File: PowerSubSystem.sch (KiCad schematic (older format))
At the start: 14 parts, among them U401 LM3671

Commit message: lib update so it only includes user-made library
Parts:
- C401, C402, C404, C405, C406, C408, C409, C410: symbol BeagleBone-Black-Cape-rescue:C-Device -> UserMade-BB-Zigbee-Gateway-CAPE:C-Device
- C403, C407: symbol BeagleBone-Black-Cape-rescue:C_Small-Device -> UserMade-BB-Zigbee-Gateway-CAPE:C_Small-Device
- FB401: symbol BeagleBone-Black-Cape-rescue:Ferrite_Bead_Small-Device -> UserMade-BB-Zigbee-Gateway-CAPE:Ferrite_Bead_Small-Device
- L401: symbol BeagleBone-Black-Cape-rescue:L_Small-Device -> UserMade-BB-Zigbee-Gateway-CAPE:L_Small-Device
- L402: symbol BeagleBone-Black-Cape-rescue:INDUCTOR-pspice -> UserMade-BB-Zigbee-Gateway-CAPE:INDUCTOR-pspice
- U401: symbol pwr_BeagleBone:LM3671 -> UserMade-BB-Zigbee-Gateway-CAPE:LM3671
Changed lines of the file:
@@
 5Vin+ Comes from the 5V output \nof the beaglebone. The one \nthat is connected to the 12V \ninput.
 $Comp
-L pwr_BeagleBone:LM3671 U401
+L UserMade-BB-Zigbee-Gateway-CAPE:LM3671 U401
 U 1 1 613D6B2B
 P 3600 6150
@@
 $EndComp
 $Comp
-L BeagleBone-Black-Cape-rescue:C_Small-Device C403
+L UserMade-BB-Zigbee-Gateway-CAPE:C_Small-Device C403
 U 1 1 613D8B5E
 P 2950 6550
@@
 	3150 6500 3150 6800
 $Comp
-L BeagleBone-Black-Cape-rescue:L_Small-Device L401
+L UserMade-BB-Zigbee-Gateway-CAPE:L_Small-Device L401
 U 1 1 613E2221
 P 4150 6300
@@
 	4350 6500 4350 6300
 $Comp
-L BeagleBone-Black-Cape-rescue:GND-power #PWR0404
+L UserMade-BB-Zigbee-Gateway-CAPE:GND-power #PWR0404
 U 1 1 613E4C24
 P 2950 6900
@@
 	2950 6900 2950 6800
 $Comp
-L BeagleBone-Black-Cape-rescue:C_Small-Device C407
+L UserMade-BB-Zigbee-Gateway-CAPE:C_Small-Device C407
 U 1 1 613E66FD
 P 4600 6550
@@
 $EndComp
 $Comp
-L BeagleBone-Black-Cape-rescue:GND-power #PWR0408
+L UserMade-BB-Zigbee-Gateway-CAPE:GND-power #PWR0408
 U 1 1 613EB575
 P 4600 6900
@@
 Connection ~ 3150 6800
 $Comp
-L pwr_BeagleBone:SYS_5V #PWR0402
+L UserMade-BB-Zigbee-Gateway-CAPE:SYS_5V #PWR0402
 U 1 1 614A8F35
 P 2600 6300
@@
 VDDR
 $Comp
-L BeagleBone-Black-Cape-rescue:C-Device C402
+L UserMade-BB-Zigbee-Gateway-CAPE:C-Device C402
 U 1 1 614ACFF1
 P 2800 2950
@@
 $EndComp
 $Comp
-L BeagleBone-Black-Cape-rescue:C-Device C401
+L UserMade-BB-Zigbee-Gateway-CAPE:C-Device C401
 U 1 1 614AD67F
 P 2300 2950
@@
 $EndComp
 $Comp
-L BeagleBone-Black-Cape-rescue:C-Device C409
+L UserMade-BB-Zigbee-Gateway-CAPE:C-Device C409
 U 1 1 614ADB54
 P 8450 2950
@@
 $EndComp
 $Comp
-L BeagleBone-Black-Cape-rescue:C-Device C406
+L UserMade-BB-Zigbee-Gateway-CAPE:C-Device C406
 U 1 1 614ADE06
 P 4350 2950
@@
 $EndComp
 $Comp
-L BeagleBone-Black-Cape-rescue:C-Device C404
+L UserMade-BB-Zigbee-Gateway-CAPE:C-Device C404
 U 1 1 614ADFDD
 P 3300 2950
@@
 $EndComp
 $Comp
-L BeagleBone-Black-Cape-rescue:C-Device C410
+L UserMade-BB-Zigbee-Gateway-CAPE:C-Device C410
 U 1 1 614AE392
 P 8950 2950
@@
 $EndComp
 $Comp
-L BeagleBone-Black-Cape-rescue:C-Device C405
+L UserMade-BB-Zigbee-Gateway-CAPE:C-Device C405
 U 1 1 614AE569
 P 3850 2950
@@
 $EndComp
 $Comp
-L BeagleBone-Black-Cape-rescue:C-Device C408
+L UserMade-BB-Zigbee-Gateway-CAPE:C-Device C408
 U 1 1 614AE740
 P 7600 2950
@@
 $EndComp
 $Comp
-L BeagleBone-Black-Cape-rescue:INDUCTOR-pspice L402
+L UserMade-BB-Zigbee-Gateway-CAPE:INDUCTOR-pspice L402
 U 1 1 614B2435
 P 7050 2800
@@
 $EndComp
 $Comp
-L BeagleBone-Black-Cape-rescue:GND-power #PWR0401
+L UserMade-BB-Zigbee-Gateway-CAPE:GND-power #PWR0401
 U 1 1 614B60EB
 P 2300 3100
@@
 $EndComp
 $Comp
-L BeagleBone-Black-Cape-rescue:GND-power #PWR0403
+L UserMade-BB-Zigbee-Gateway-CAPE:GND-power #PWR0403
 U 1 1 614B633D
 P 2800 3100
@@
 $EndComp
 $Comp
-L BeagleBone-Black-Cape-rescue:GND-power #PWR0405
+L UserMade-BB-Zigbee-Gateway-CAPE:GND-power #PWR0405
 U 1 1 614B6607
 P 3300 3100
@@
 $EndComp
 $Comp
-L BeagleBone-Black-Cape-rescue:GND-power #PWR0406
+L UserMade-BB-Zigbee-Gateway-CAPE:GND-power #PWR0406
 U 1 1 614B68D5
 P 3850 3100
@@
 $EndComp
 $Comp
-L BeagleBone-Black-Cape-rescue:GND-power #PWR0407
+L UserMade-BB-Zigbee-Gateway-CAPE:GND-power #PWR0407
 U 1 1 614B6CF8
 P 4350 3100
@@
 $EndComp
 $Comp
-L BeagleBone-Black-Cape-rescue:GND-power #PWR0409
+L UserMade-BB-Zigbee-Gateway-CAPE:GND-power #PWR0409
 U 1 1 614B73B7
 P 7600 3100
@@
 $EndComp
 $Comp
-L BeagleBone-Black-Cape-rescue:GND-power #PWR0410
+L UserMade-BB-Zigbee-Gateway-CAPE:GND-power #PWR0410
 U 1 1 614B76A1
 P 8450 3100
@@
 $EndComp
 $Comp
-L BeagleBone-Black-Cape-rescue:GND-power #PWR0411
+L UserMade-BB-Zigbee-Gateway-CAPE:GND-power #PWR0411
 U 1 1 614B7948
 P 8950 3100
@@
 MCU_VDD
 $Comp
-L BeagleBone-Black-Cape-rescue:Ferrite_Bead_Small-Device FB401
+L UserMade-BB-Zigbee-Gateway-CAPE:Ferrite_Bead_Small-Device FB401
 U 1 1 614B96C9
 P 2000 2800

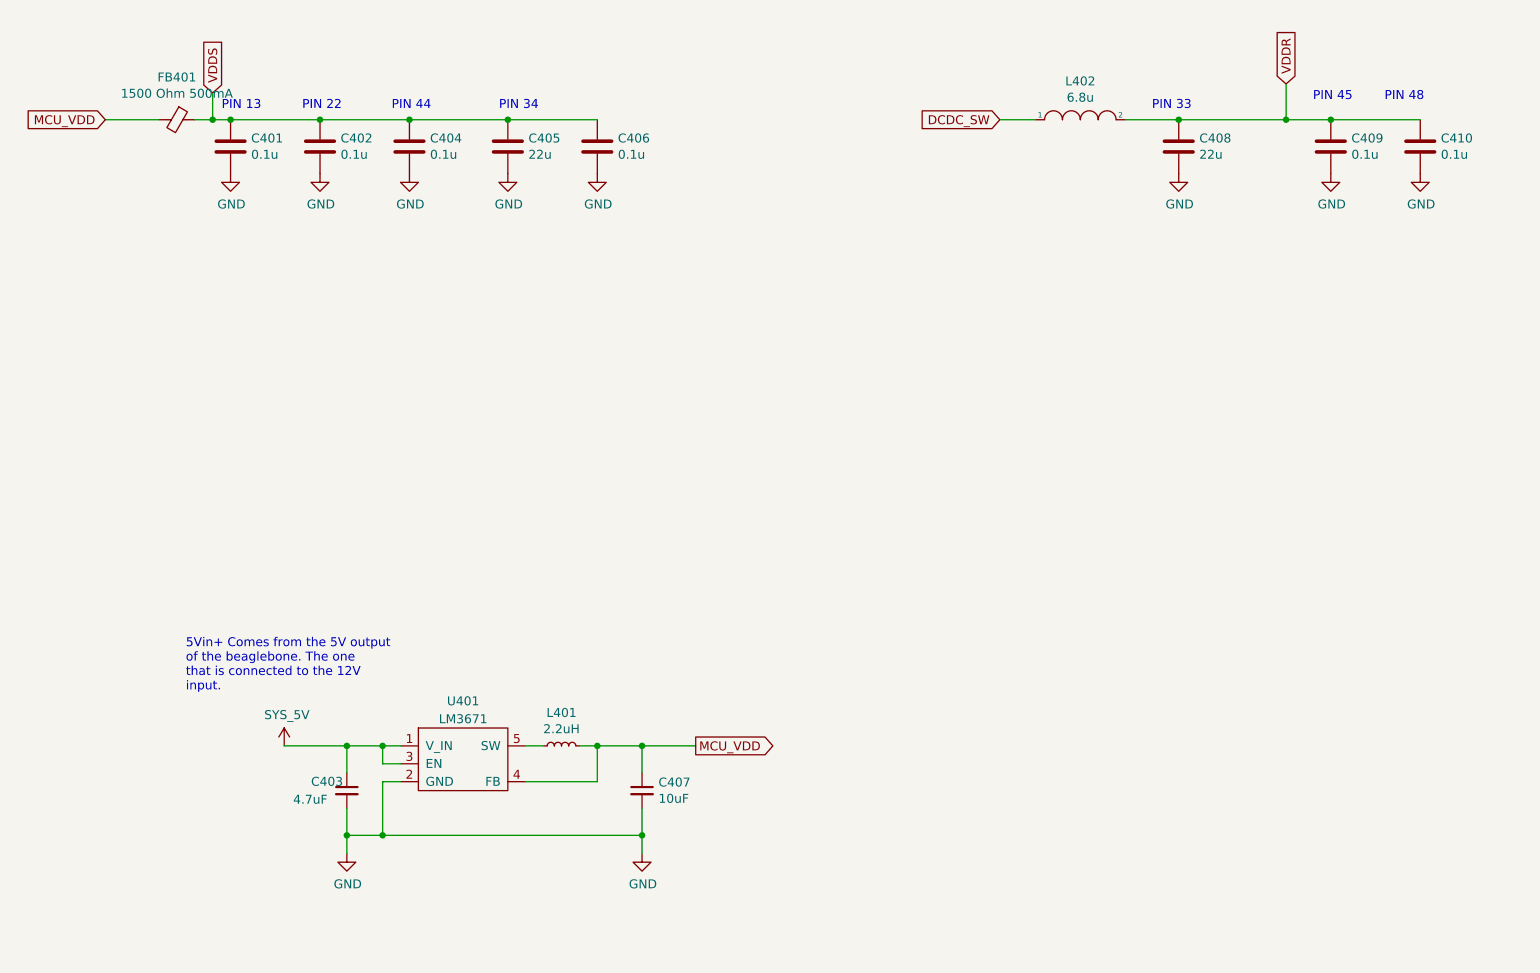
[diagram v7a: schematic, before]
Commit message: final edits before it'll be untouched
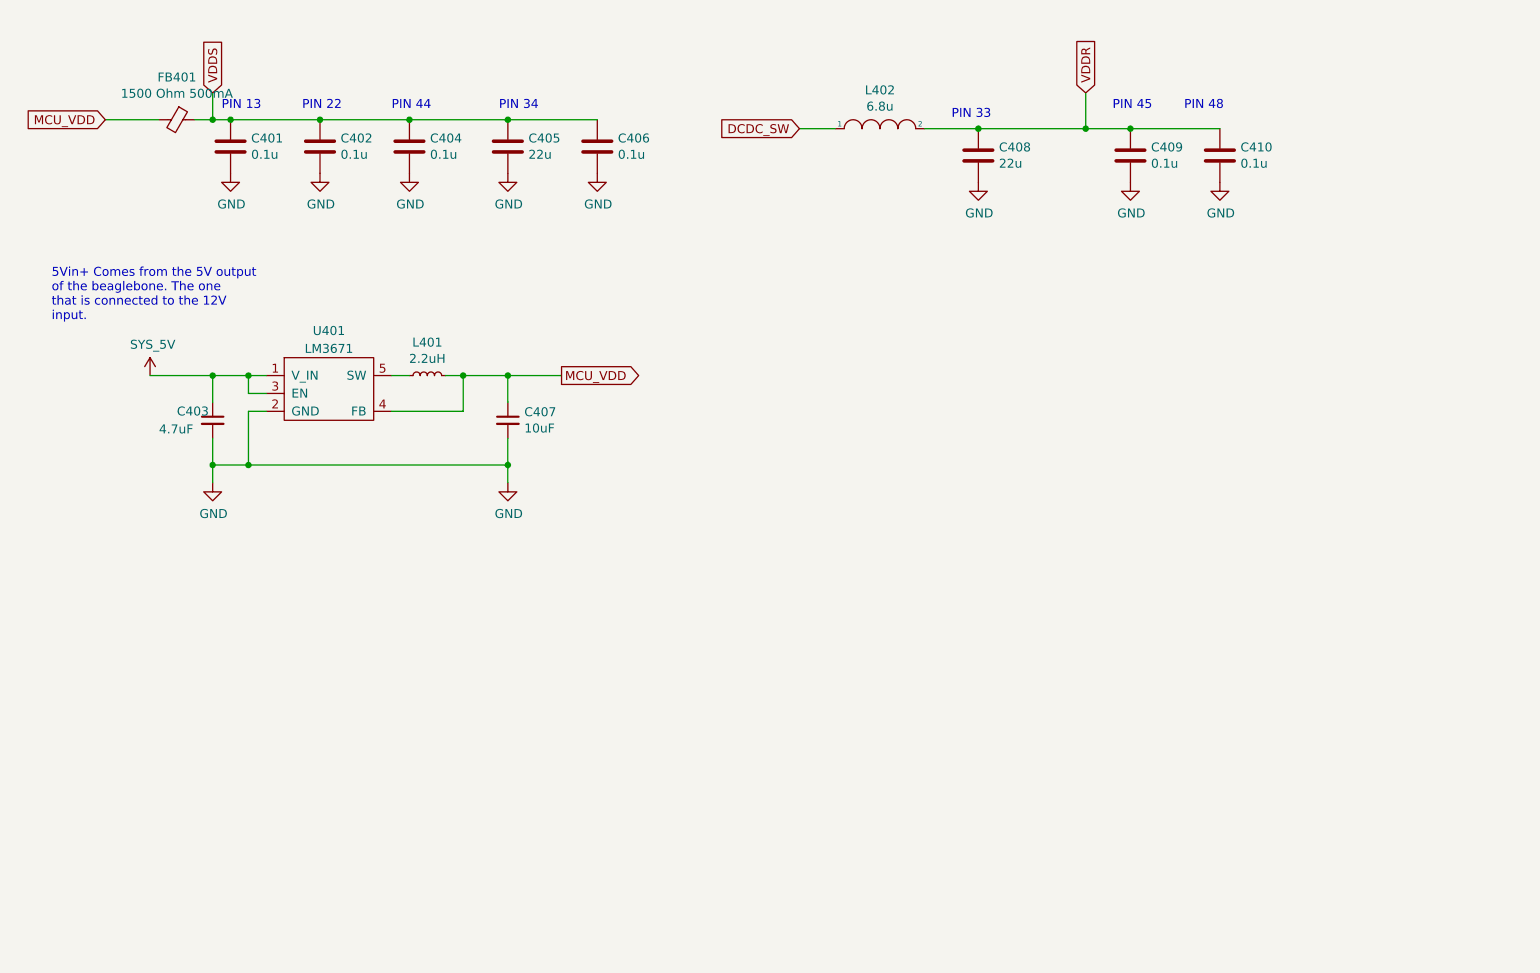
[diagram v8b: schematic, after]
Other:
- moved on the sheet: C403, C407, C408, C409, C410, L401, L402, U401
